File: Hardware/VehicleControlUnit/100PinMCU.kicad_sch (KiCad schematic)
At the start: 33 parts, among them J10 SWD_Header, J11 SWD, SW1 SW_SPDT, U4 STM32G473VETx, Y1 Crystal

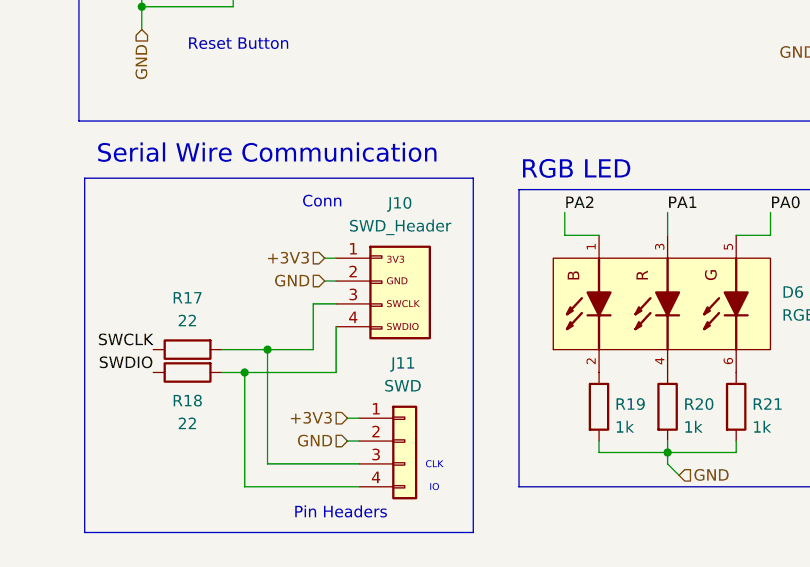
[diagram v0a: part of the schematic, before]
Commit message: VCU hardware prod files done night night
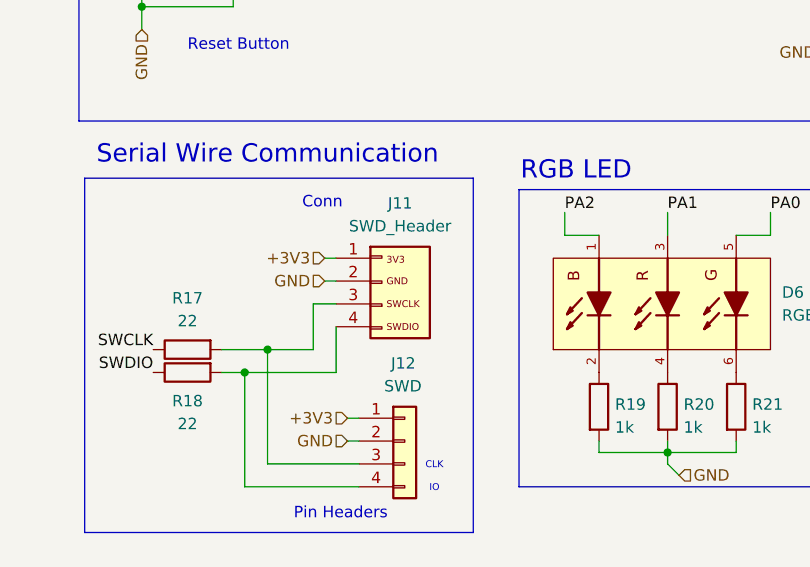
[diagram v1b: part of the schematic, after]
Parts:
- renumbered J10 to J11, J11 to J12
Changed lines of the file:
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@@
 		(in_pos_files yes)
 		(dnp no)
-		(property "Reference" "J10"
+		(property "Reference" "J11"
 			(at 225.552 128.524 0)
 			(show_name no)
@@
 			(project "VehicleControlUnit"
 				(path "/e864fac9-3897-46c9-9101-6d5488c6cd3a/f9087b5b-32fd-4bb7-84dd-9fe64614d383/e8918db0-ed0e-4663-8139-dd25306e146c"
-					(reference "J10")
+					(reference "J11")
 					(unit 1)
 				)
@@
 		(in_pos_files yes)
 		(dnp no)
-		(property "Reference" "J11"
+		(property "Reference" "J12"
 			(at 224.536 146.304 0)
 			(show_name no)
@@
 			(project "VehicleControlUnit"
 				(path "/e864fac9-3897-46c9-9101-6d5488c6cd3a/f9087b5b-32fd-4bb7-84dd-9fe64614d383/e8918db0-ed0e-4663-8139-dd25306e146c"
-					(reference "J11")
+					(reference "J12")
 					(unit 1)
 				)

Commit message: surabhi review pls
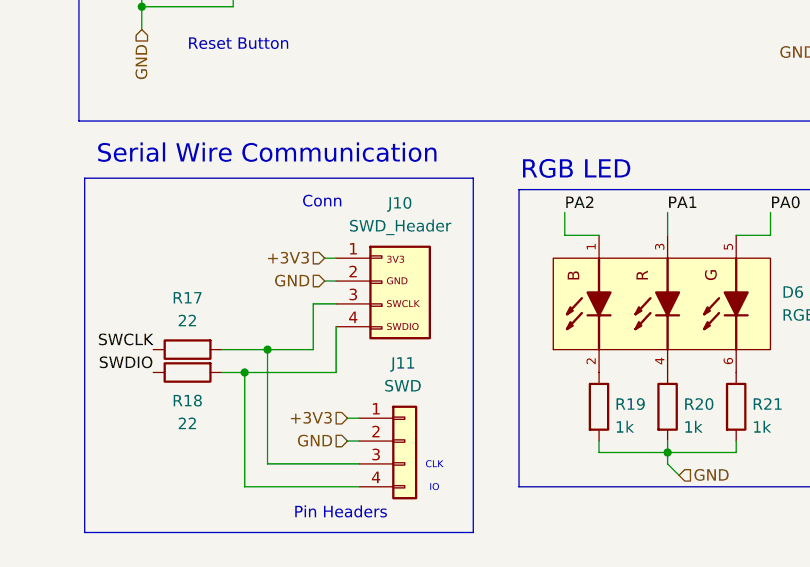
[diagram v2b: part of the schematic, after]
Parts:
- renumbered J11 to J10, J12 to J11
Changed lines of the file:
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@@
 		(in_pos_files yes)
 		(dnp no)
-		(property "Reference" "J11"
+		(property "Reference" "J10"
 			(at 225.552 128.524 0)
 			(show_name no)
@@
 			(project "VehicleControlUnit"
 				(path "/e864fac9-3897-46c9-9101-6d5488c6cd3a/f9087b5b-32fd-4bb7-84dd-9fe64614d383/e8918db0-ed0e-4663-8139-dd25306e146c"
-					(reference "J11")
+					(reference "J10")
 					(unit 1)
 				)
@@
 		(in_pos_files yes)
 		(dnp no)
-		(property "Reference" "J12"
+		(property "Reference" "J11"
 			(at 224.536 146.304 0)
 			(show_name no)
@@
 			(project "VehicleControlUnit"
 				(path "/e864fac9-3897-46c9-9101-6d5488c6cd3a/f9087b5b-32fd-4bb7-84dd-9fe64614d383/e8918db0-ed0e-4663-8139-dd25306e146c"
-					(reference "J12")
+					(reference "J11")
 					(unit 1)
 				)
